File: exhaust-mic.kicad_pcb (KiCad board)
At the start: 4 copper layers, 72 x 55 mm, 131 parts, among them J1 XH-6pol_Power_CAN, J2 XH-5pol_MicA, J3 XH-5pol_MicB, J4 USB-C, J5 microSD_PushPush, J6 GPS_unbestueckt, J7 I2C_Erweiterung, Q1 ZXMP6A17E6, Q3 2N7002, Q4 2N7002, SW1 RESET, SW2 BOOT, SW3 REC, SW4 MARK, U1 LM5164DDA, U2 TLV1117LV33, U3 TPS7A2033, U5 PCM1863DBT, U6 ESP32-S3-WROOM-1-N8R2, U7 DS3231SN, U8 SN65HVD230D, Y1 24.576MHz

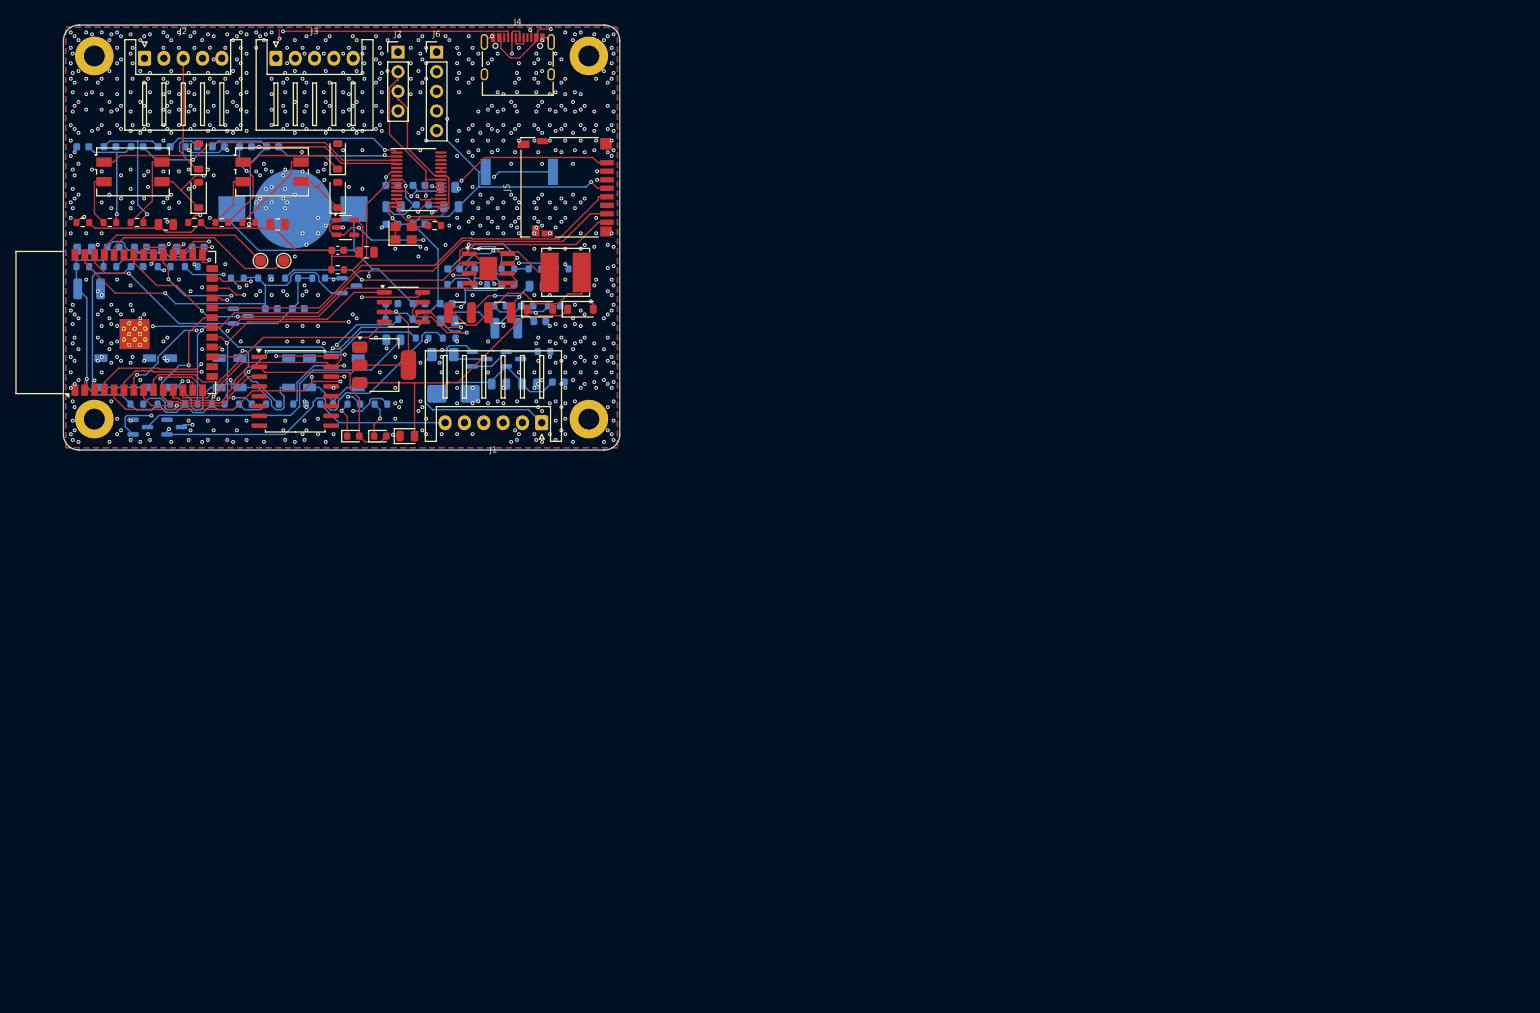
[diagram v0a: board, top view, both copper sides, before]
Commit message: modified:   01-power.kicad_sch 	modified:   02-analog.kicad_sch 	modified:   03-adc.kicad_sch 	modified:   04-mcu.kicad_sch 	modified:   05-io.kicad_sch 	modified:   exhaust-mic.kicad_pcb 	modified:   exhaust-mic.kicad_pro 	modified:   exhaust-mic.kicad_sch 	modified:   mic-head/mic-head.kicad_pcb 	modified:   mic-head/mic-head.kicad_pro 	modified:   mic-head/mic-head.kicad_sch 	new file:   ~exhaust-mic.kicad_pro.lck
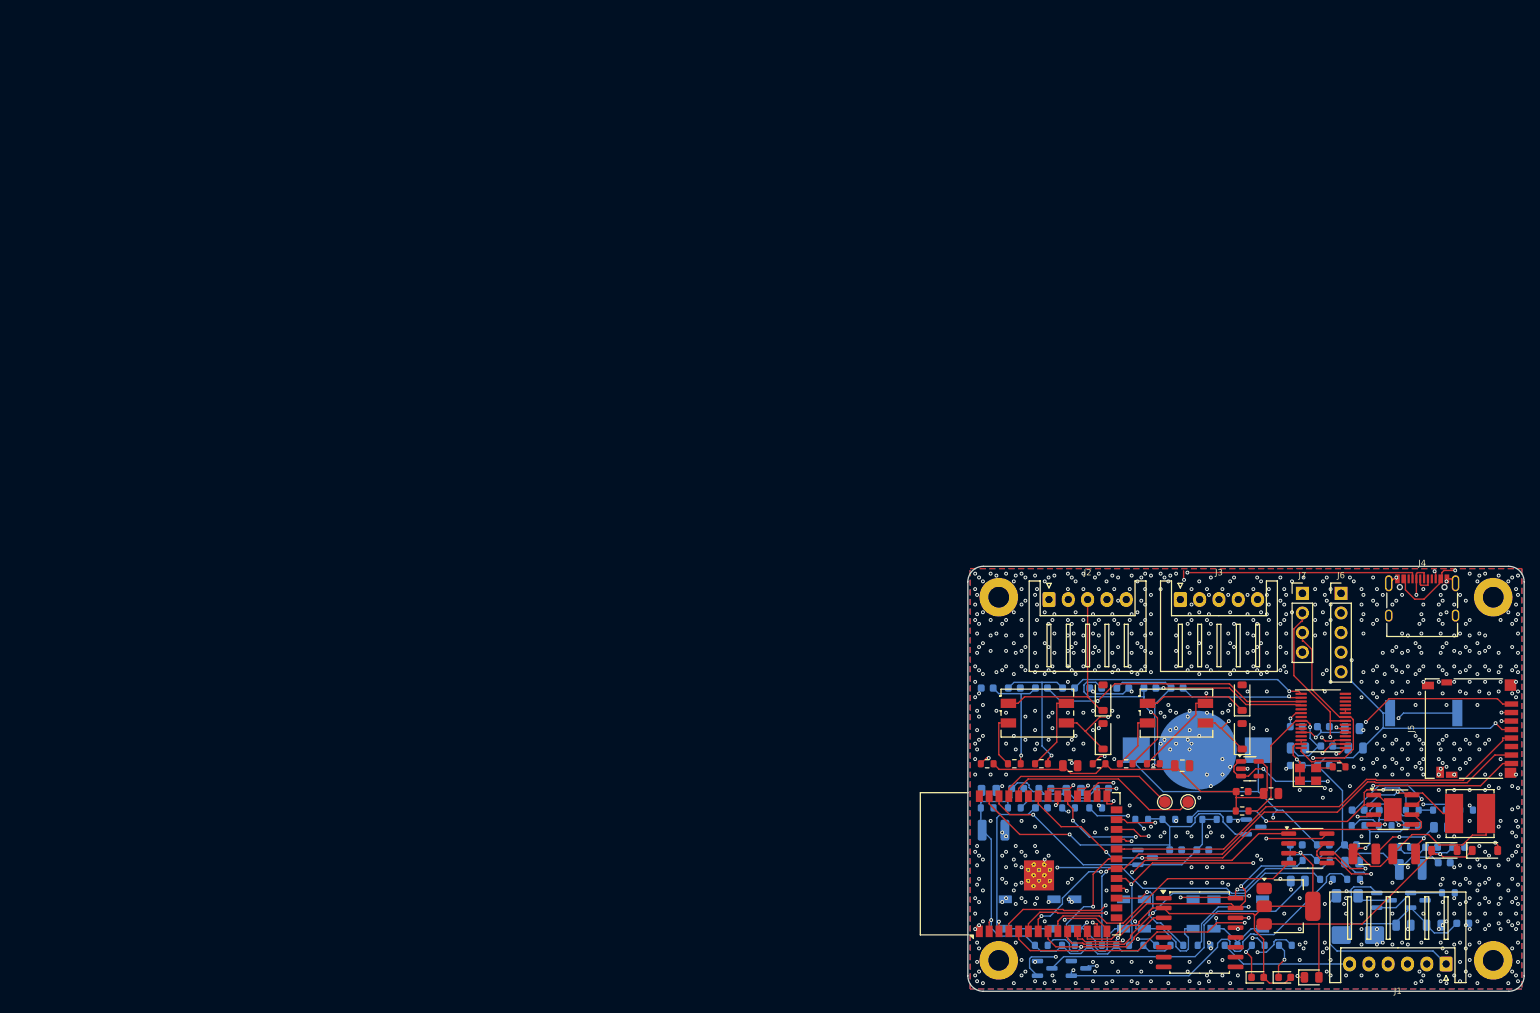
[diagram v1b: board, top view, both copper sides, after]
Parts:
- moved C1 136.4 mm to (173.4, 116.5)
- moved C12 136.4 mm to (178.7, 108.4)
- moved C14 136.4 mm to (152.6, 99.2)
- moved C20 136.4 mm to (130.3, 95.9)
- moved C21 136.4 mm to (119.6, 85.8)
- moved C23 136.4 mm to (126.6, 85.8)
- moved C24 136.4 mm to (130.1, 85.8)
- moved C28 136.4 mm to (140.6, 85.8)
- moved C29 136.4 mm to (144.1, 85.8)
- moved C30 136.4 mm to (159.6, 90.8)
- moved C33 136.4 mm to (159.8, 93.6)
- moved C35 136.4 mm to (167.2, 93.6)
- moved C36 136.4 mm to (159.6, 95.8)
- moved C4 136.4 mm to (167.6, 101.6)
- moved C41 136.4 mm to (119.8, 99.1)
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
